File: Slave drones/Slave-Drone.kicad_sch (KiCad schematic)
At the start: 41 parts, among them J1 Conn_01x02, J2 Conn_01x02, J3 Conn_01x02, J4 Conn_01x02, J5 USB_C_Receptacle_USB2.0_16P, J6 Conn_01x02, SW1 SW_Push, SW2 SW_Push, U1 MPU6500, U2 QMC5883L, U3 ESP32-S3-MINI-1, U4 AP2112K-3.3

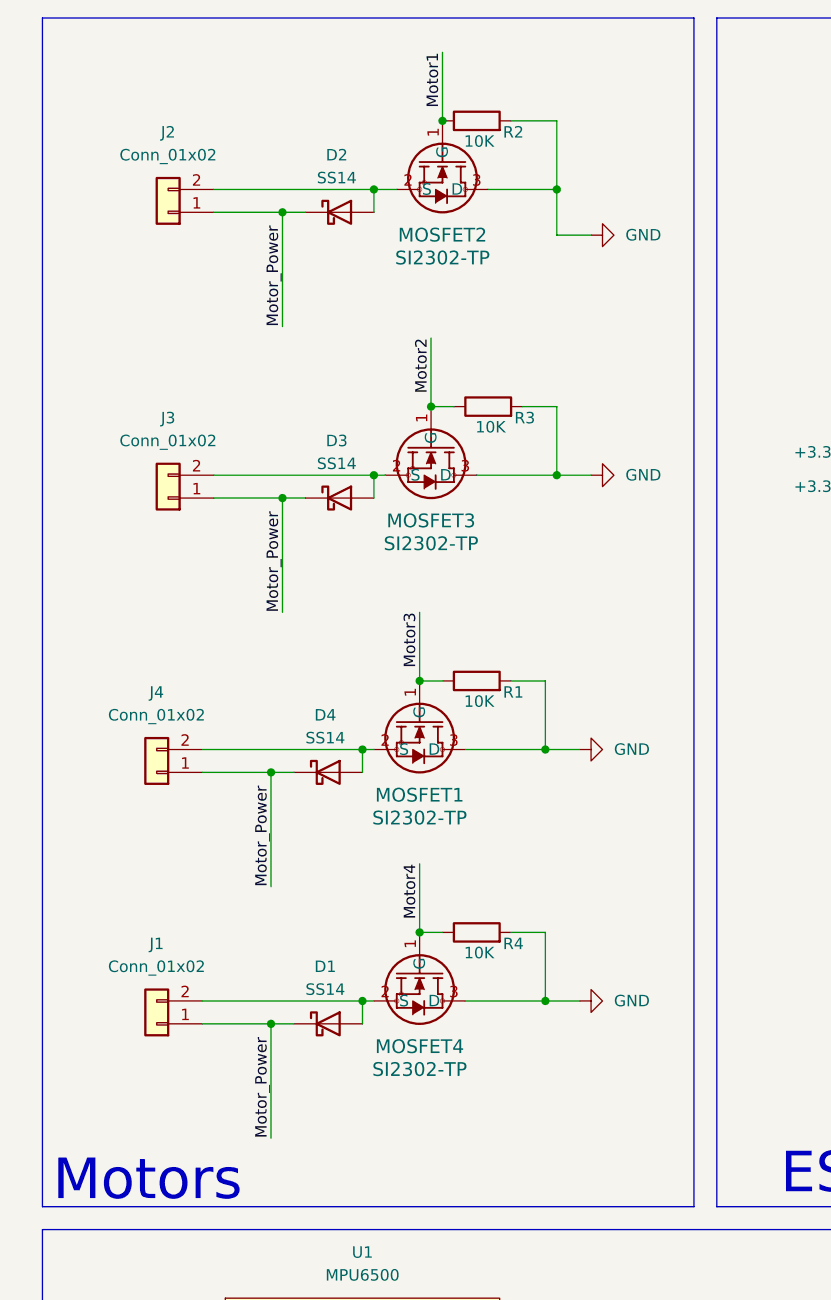
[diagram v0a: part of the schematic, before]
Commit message: nothing
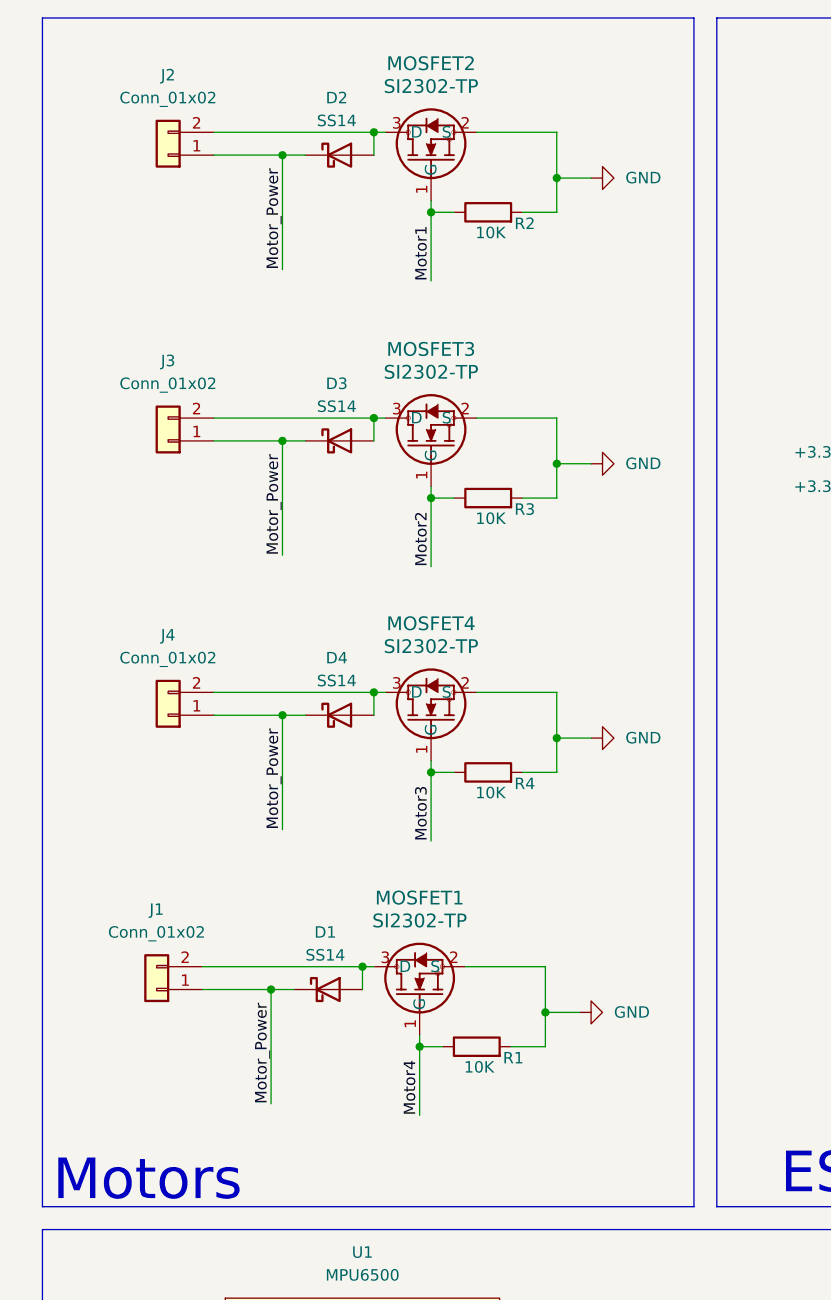
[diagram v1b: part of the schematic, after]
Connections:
- net GND: now also MOSFET1.2 (S), MOSFET2.2 (S), MOSFET3.2 (S), MOSFET4.2 (S); no longer MOSFET1.3 (D), MOSFET2.3 (D), MOSFET3.3 (D), MOSFET4.3 (D)
- net Motor3: now also MOSFET4.1 (G), R4.1; no longer MOSFET1.1 (G), R1.1
- net Motor4: now also MOSFET1.1 (G), R1.1; no longer MOSFET4.1 (G), R4.1
- net at D4.2 (A), J4.2 (Pin_2): now also MOSFET4.3 (D); no longer MOSFET1.2 (S)
- net at D2.2 (A), J2.2 (Pin_2): now also MOSFET2.3 (D); no longer MOSFET2.2 (S)
- net at D3.2 (A), J3.2 (Pin_2): now also MOSFET3.3 (D); no longer MOSFET3.2 (S)
- net at D1.2 (A), J1.2 (Pin_2): now also MOSFET1.3 (D); no longer MOSFET4.2 (S)
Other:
- moved on the sheet: D2, D3, J1, J2, J3, J4, MOSFET2, MOSFET3, R2, R3
